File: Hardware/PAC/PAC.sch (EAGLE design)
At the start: 19 parts, among them Q1 BC817, U3 DF06S

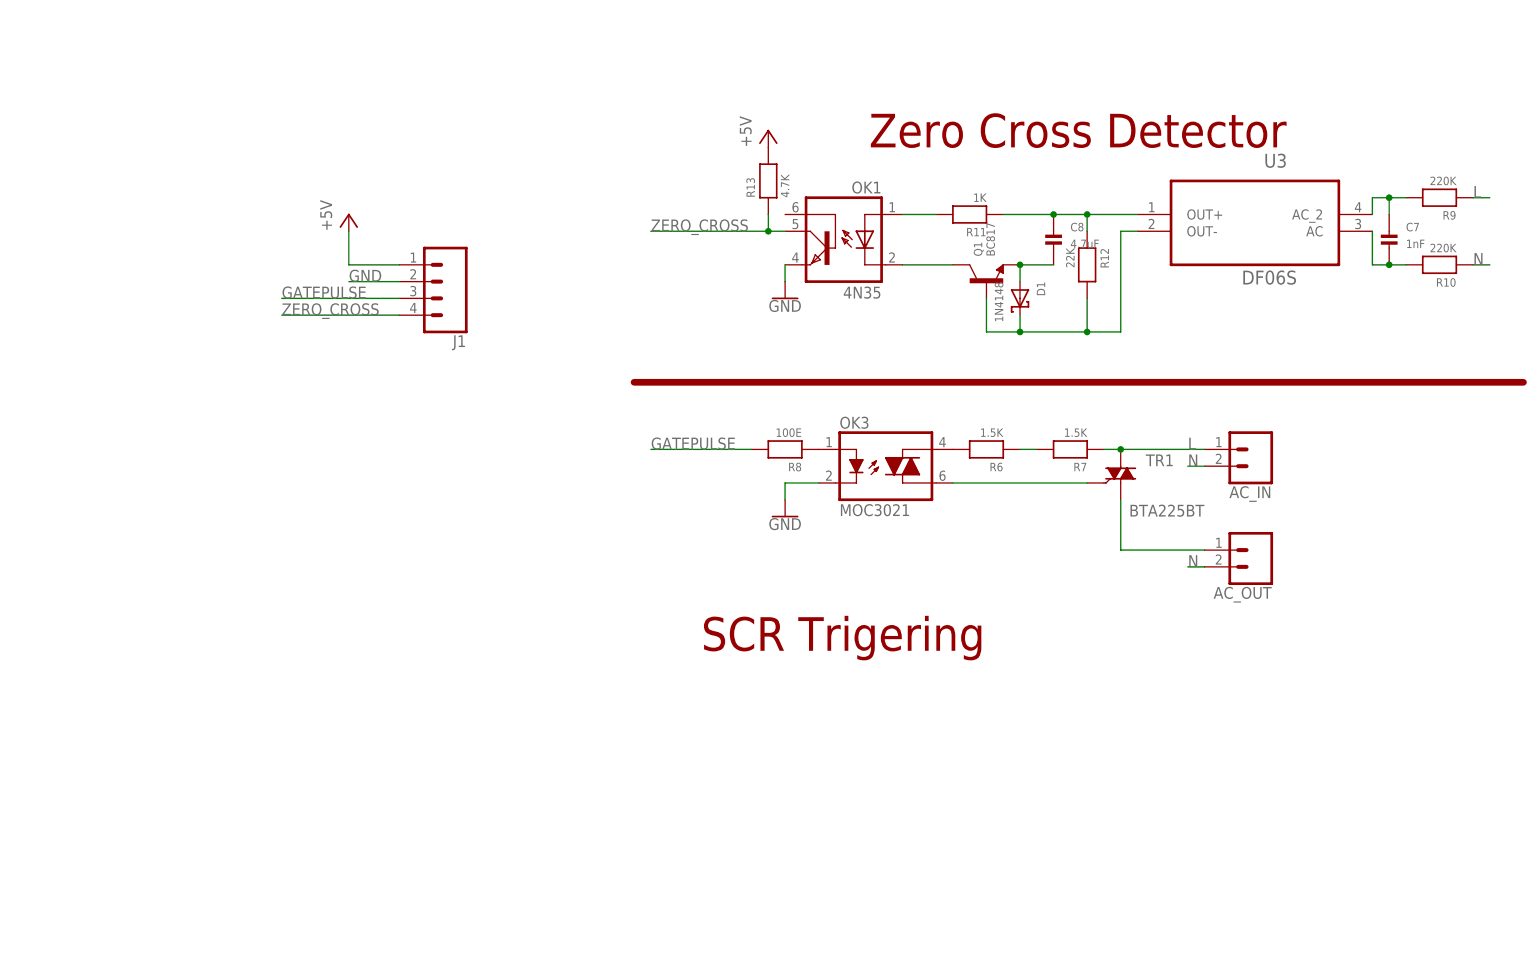
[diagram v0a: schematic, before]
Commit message: PhaseAngleControl
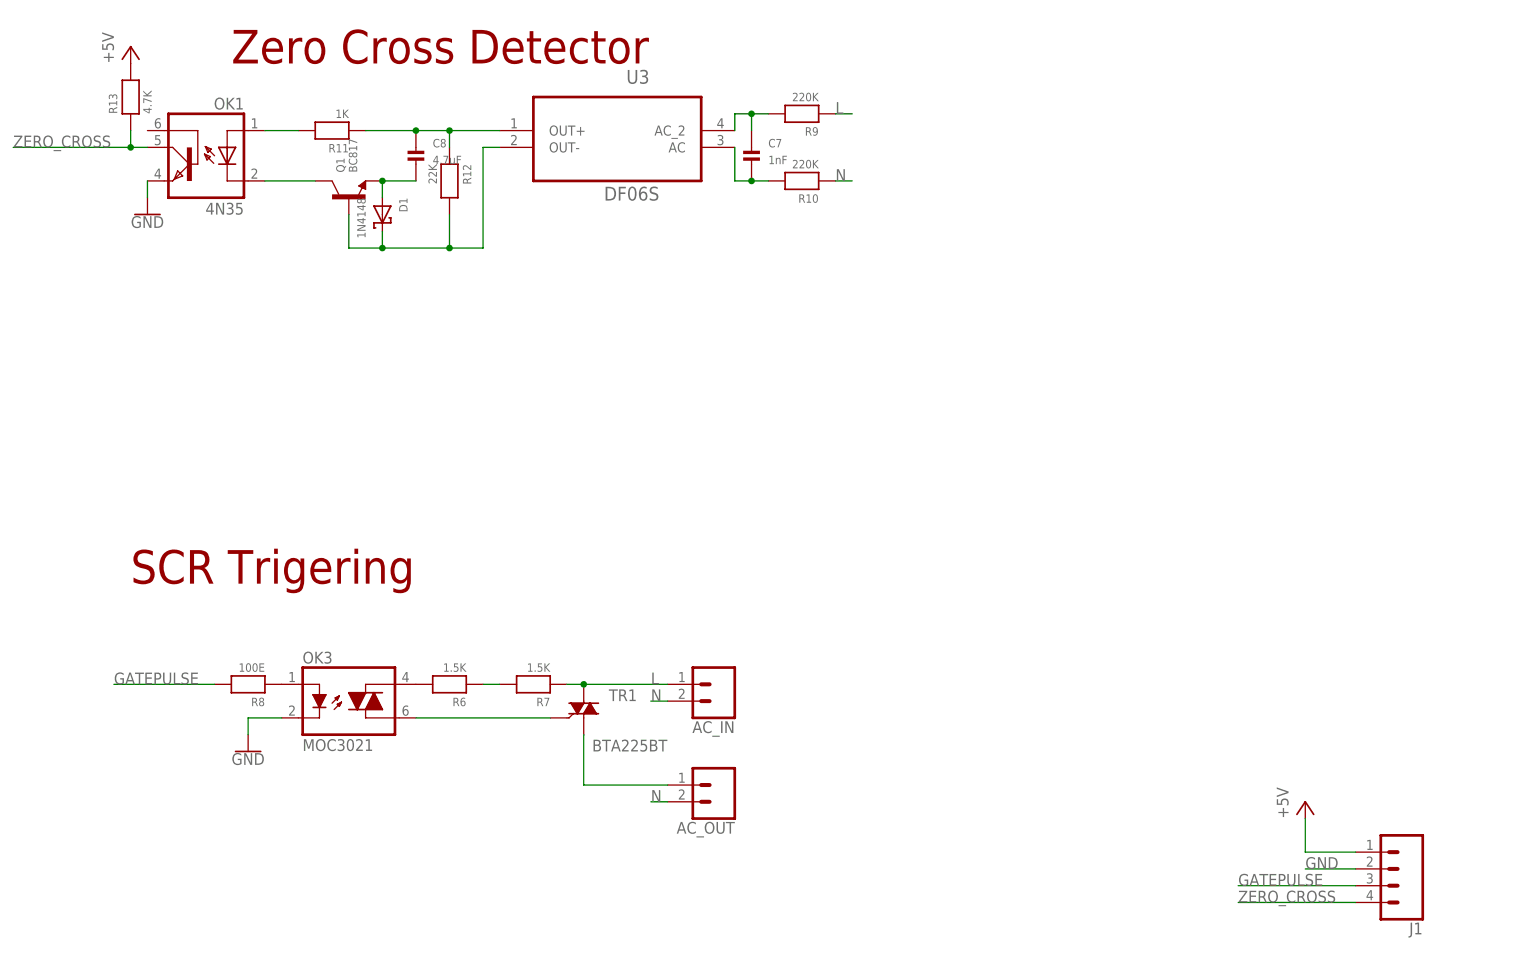
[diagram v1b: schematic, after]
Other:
- moved on the sheet: AC_IN, AC_OUT, C7, C8, D1, J1, OK1, OK3, Q1, R10, R11, R12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
